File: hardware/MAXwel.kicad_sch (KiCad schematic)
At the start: 155 parts, among them J1 Conn_02x05_Odd_Even, J2 Conn_02x12_Counter_Clockwise, J3 Barrel_Jack_Switch_Pin3Ring, SW1 SW_Push_Dual, SW10 SW_Wuerth_450301014042, SW11 SW_Wuerth_450301014042, SW12 SW_Wuerth_450301014042, SW13 SW_Wuerth_450301014042, SW2 SW_Push_Dual, SW3 SW_Push_Dual, SW4 SW_Push_Dual, SW5 SW_Wuerth_450301014042, SW6 SW_Wuerth_450301014042, SW7 SW_Wuerth_450301014042, SW8 SW_Wuerth_450301014042, SW9 SW_Push_DPDT, U1 D168K, U2 D168K, U3 D168K, U4 D168K, U5 EPM240T100, U6 AMS1117-3.3, X1 50.000, X2 14.756

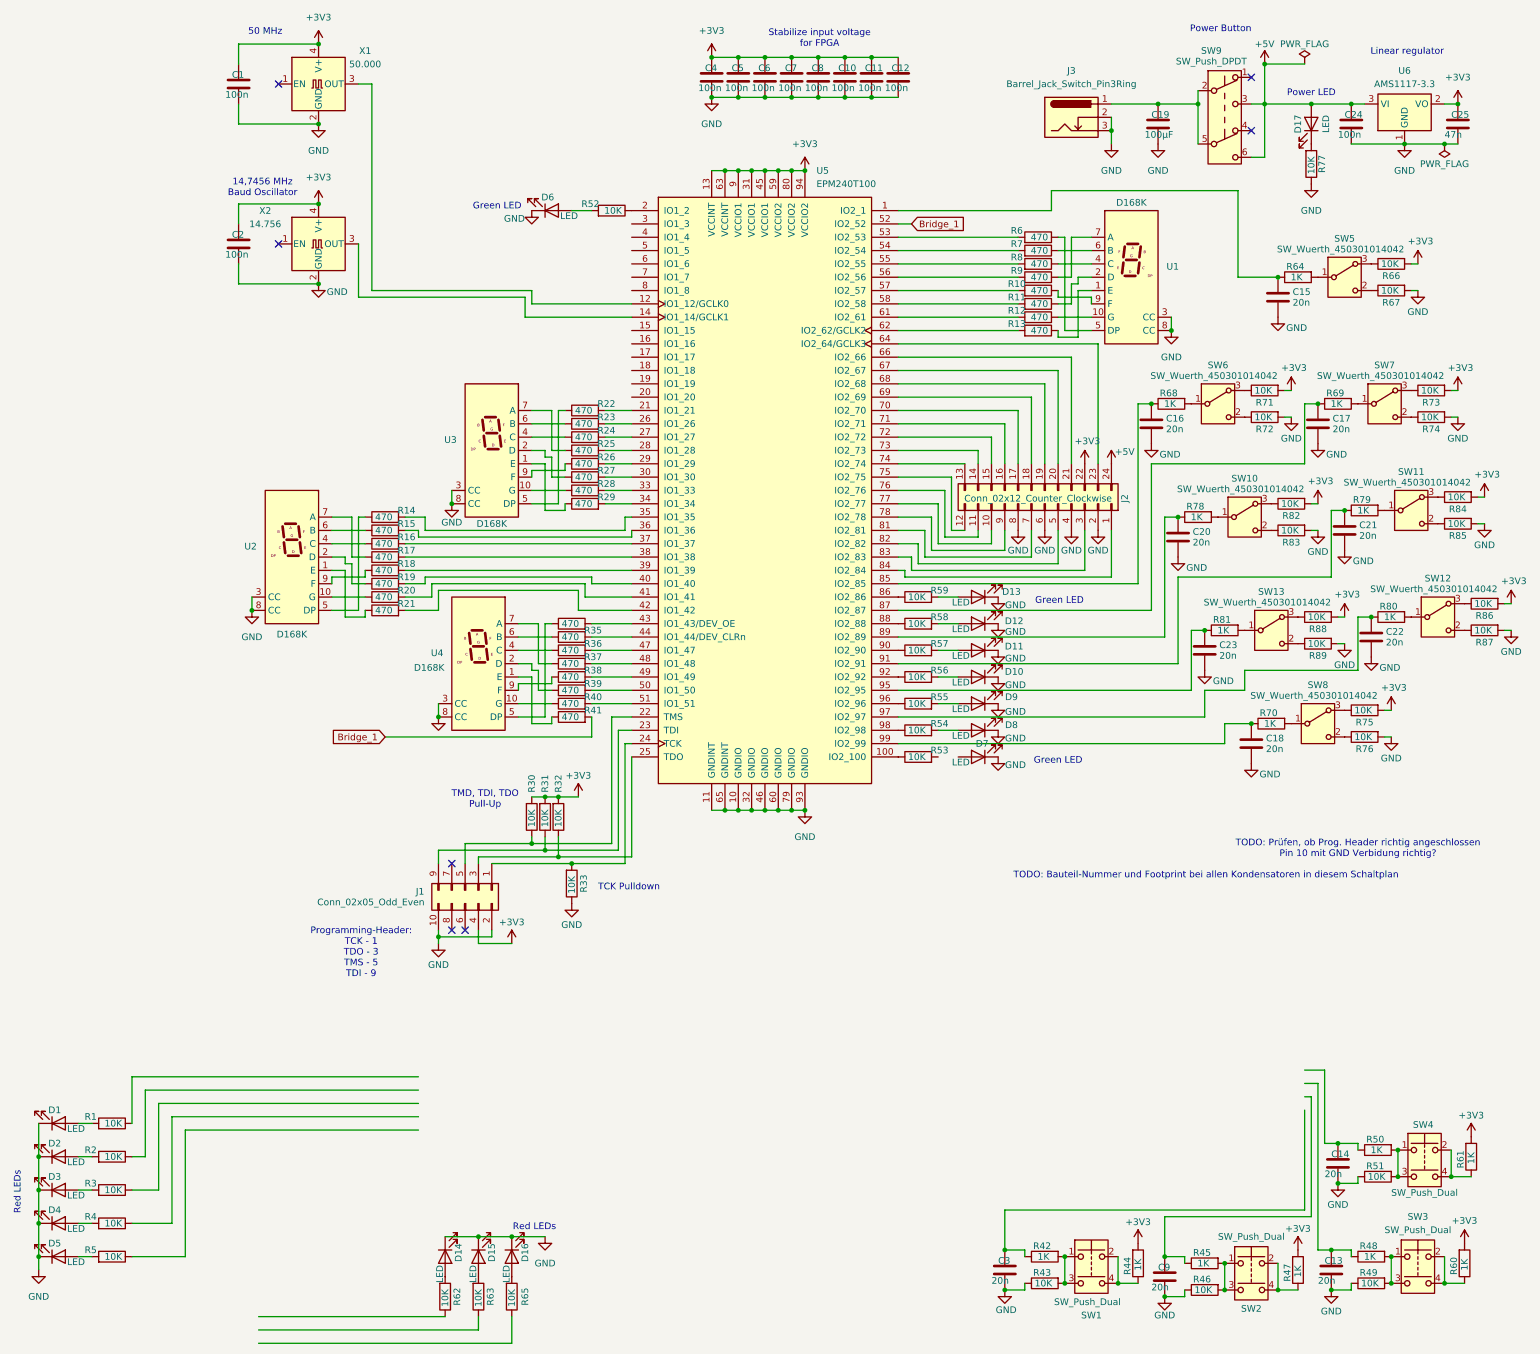
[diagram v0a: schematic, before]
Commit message: first successfull redesign
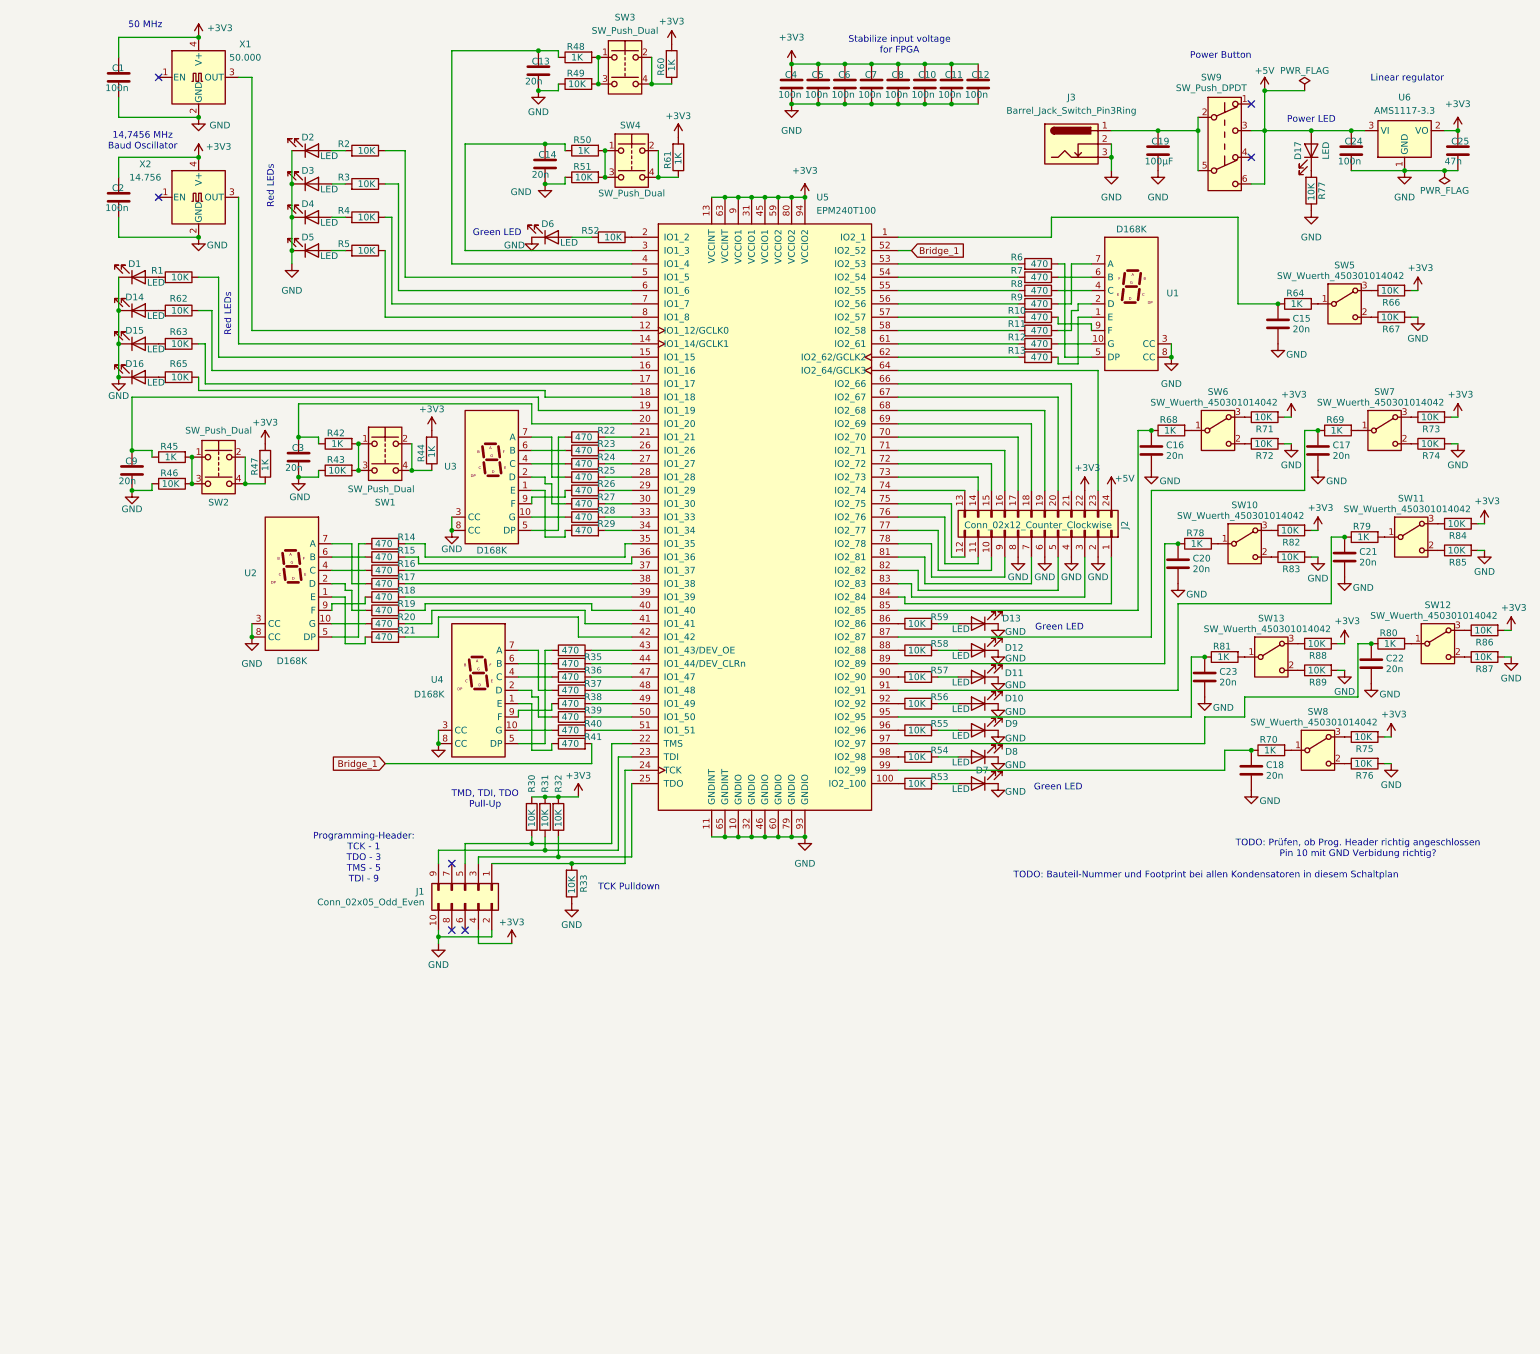
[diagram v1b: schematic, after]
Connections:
- net at C3.1, R42.1: now also U5.20 (IO1_20)
- net at R1.1: now also U5.15 (IO1_15)
- net at U5.16 (IO1_16): now also R62.1
- net at U5.17 (IO1_17): now also R63.1
- net at U5.18 (IO1_18): now also R65.1
- net at U5.19 (IO1_19): now also C9.1, R45.1
- net at U5.3 (IO1_3): now also C14.1, R50.1
- net at U5.4 (IO1_4): now also C13.1, R48.1
- net at U5.5 (IO1_5): now also R2.1
- net at U5.6 (IO1_6): now also R3.1
- net at U5.7 (IO1_7): now also R4.1
- net at U5.8 (IO1_8): now also R5.1
- net at D7.2 (A): now also R53.2
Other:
- moved on the sheet: C1, C10, C11, C12, C13, C14, C15, C16, C17, C18, C19, C2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
